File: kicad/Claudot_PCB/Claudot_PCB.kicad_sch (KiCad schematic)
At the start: 56 parts, among them J1 TYPE-C-31-M-12, SW1 SW_Push, SW10 SW_Push, SW11 SW_Push, SW12 RotaryEncoder, SW2 SW_Push, SW3 SW_Push, SW4 SW_Push, SW5 SW_Push, SW6 SW_Push, SW7 SW_Push, SW8 SW_Push, SW9 SW_Push, U1 RP2040, U2 W25Q16JVUXIQ, U3 AP2112K-3.3, Y1 12MHz

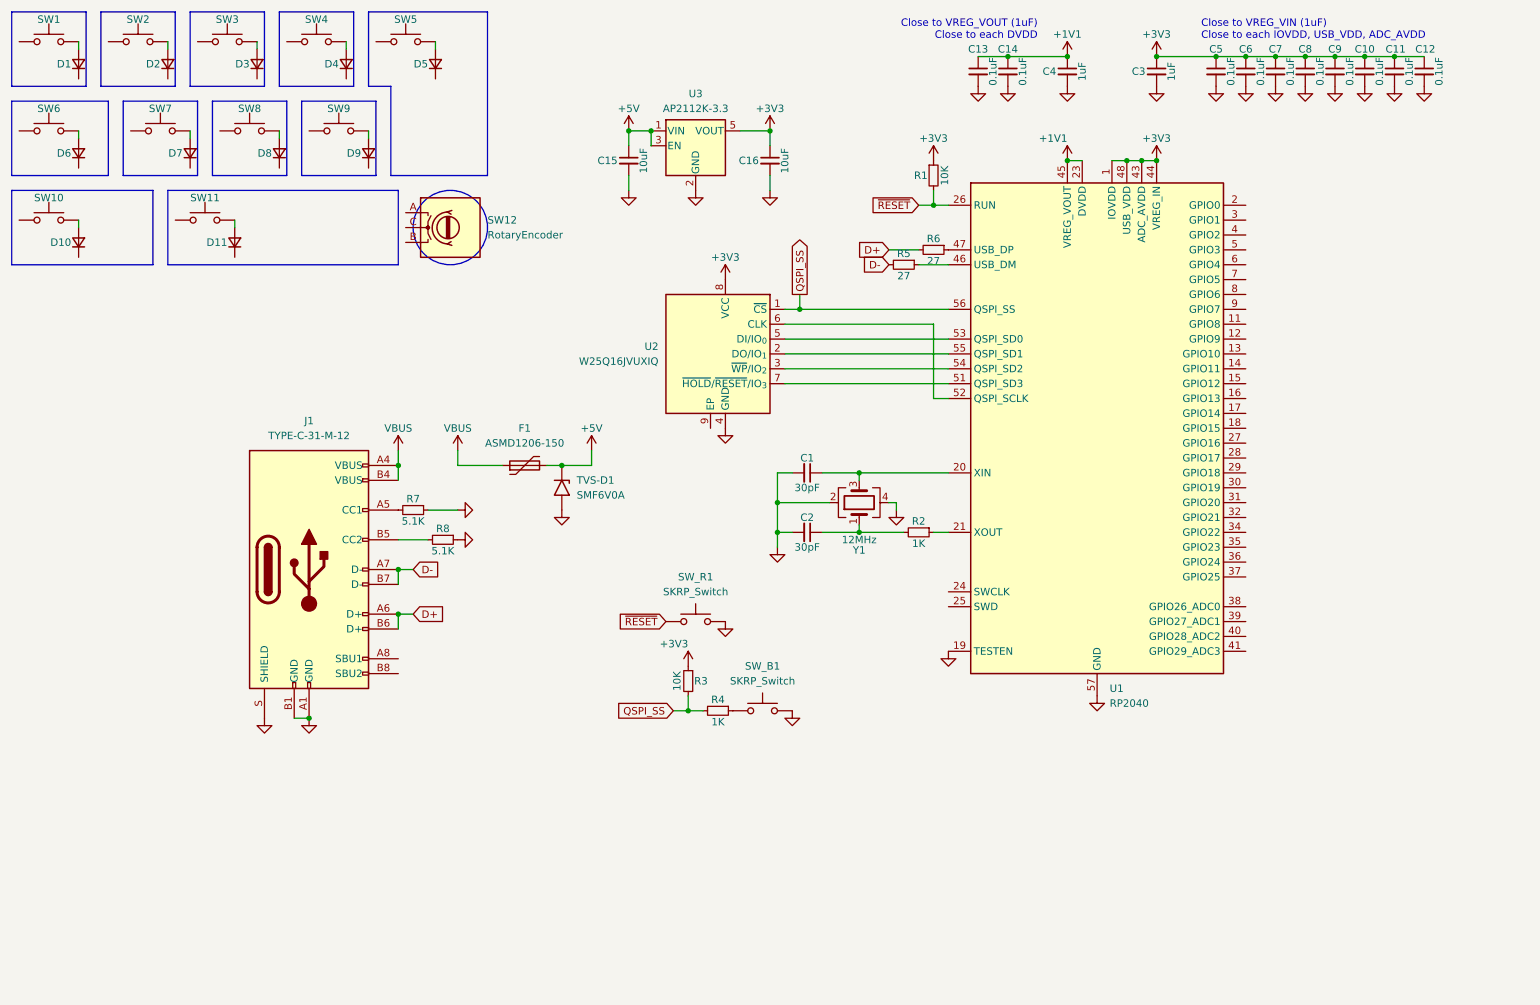
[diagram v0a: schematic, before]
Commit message: Update schematic and pcb
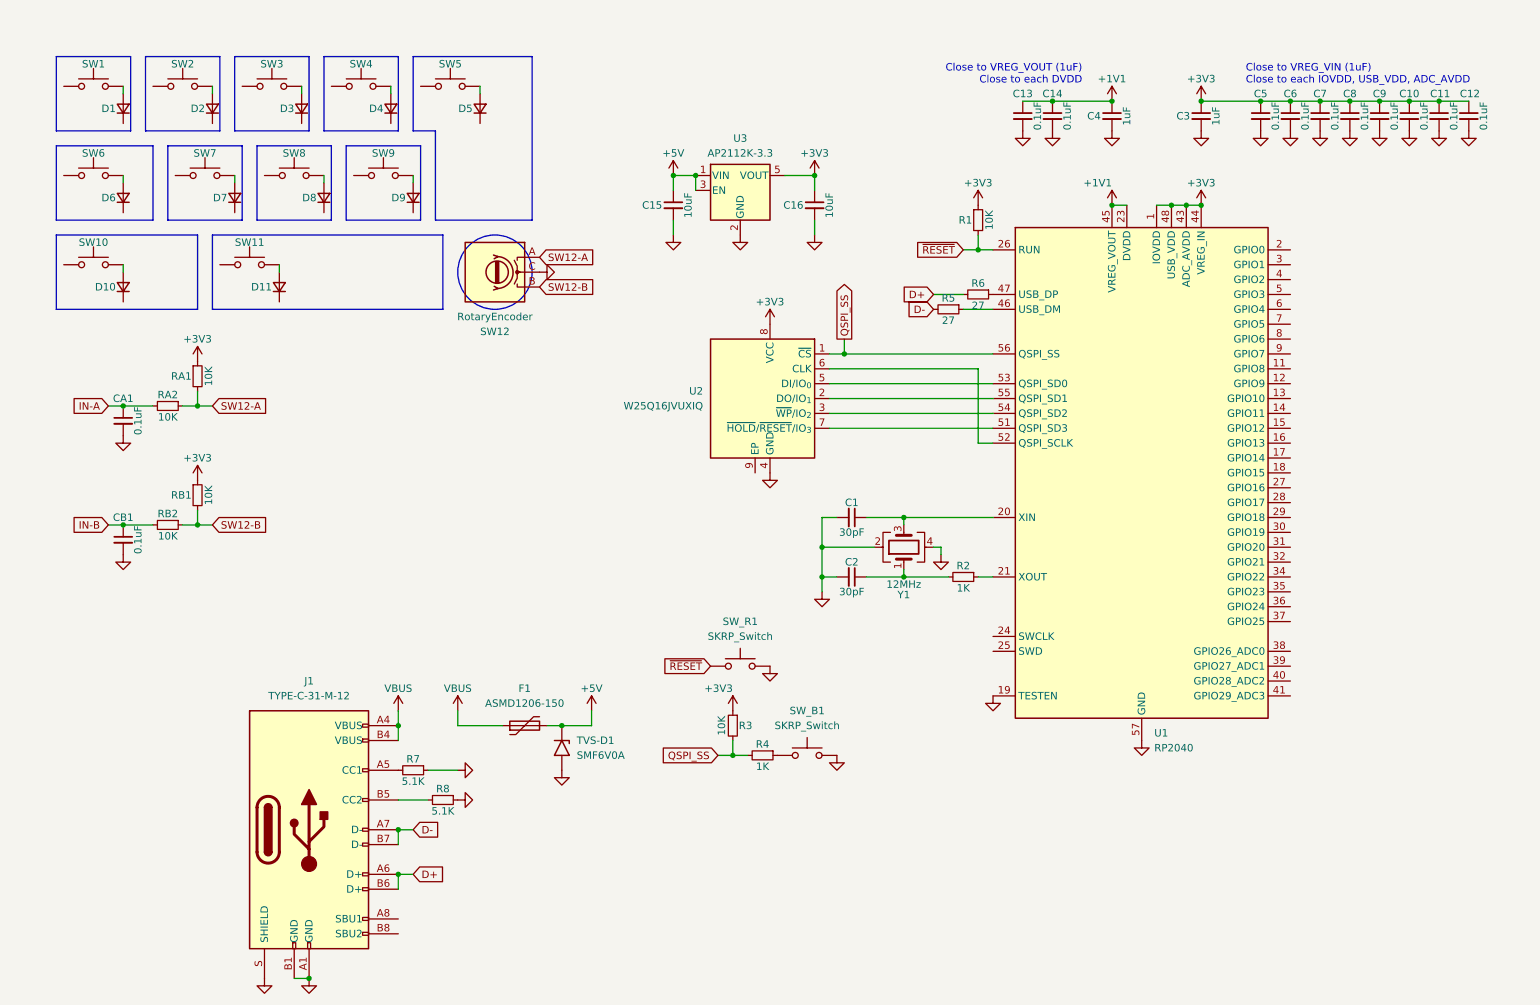
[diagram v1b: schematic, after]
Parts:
- added CA1, CB1: 0.1uF, Library:C_0402, symbol Device:C_Small
- added RA1, RA2, RB1, RB2: 10K, Library:R_0402, symbol Device:R_Small
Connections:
- net +3V3: now also RA1.1, RB1.1
- net GND: now also SW12.C, CA1.2, CB1.2
- net SW12-A: now reaches SW12.A
- net SW12-A: now also RA1.2, RA2.1
- net SW12-B: now reaches SW12.B
- net SW12-B: now also RB1.2, RB2.1
- new net IN-A: CA1.1, RA2.2
- new net IN-B: CB1.1, RB2.2
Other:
- moved on the sheet: C1, C10, C11, C12, C13, C14, C15, C16, C2, C3, C4, C5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

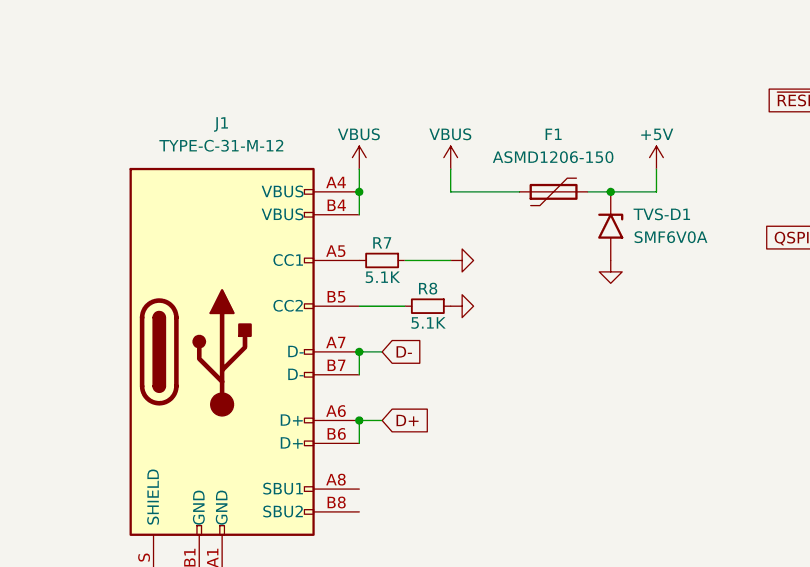
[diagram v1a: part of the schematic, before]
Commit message: Update schematic and pcb
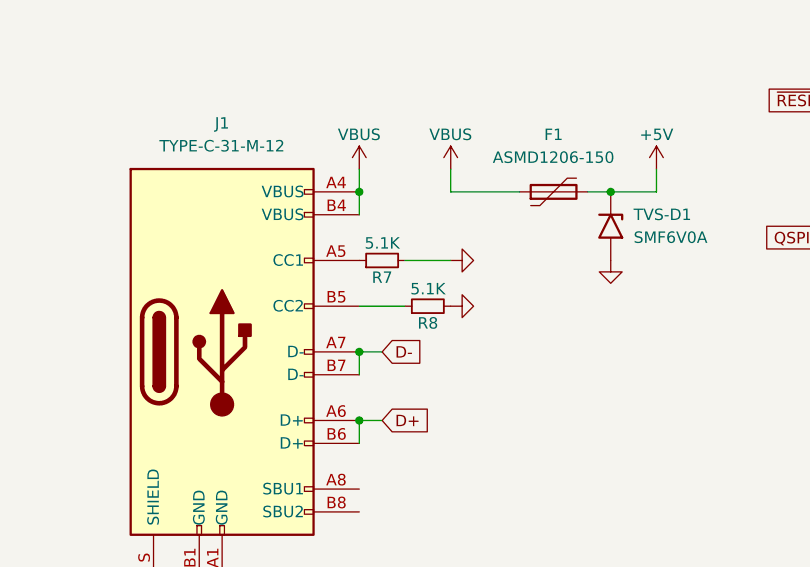
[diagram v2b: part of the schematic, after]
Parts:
- F1: footprint Fuse:Fuse_1206_3216Metric -> Library:F_1206
- TVS-D1: footprint Diode_SMD:D_SMF -> Library:SMF6.0A; LCSC (none) -> C178260
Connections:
- net GND: now also R7.2, R8.2; no longer R7.1, R8.1
- net at J1.A5 (CC1): now also R7.1; no longer R7.2
- net at J1.B5 (CC2): now also R8.1; no longer R8.2
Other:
- moved on the sheet: R7, R8
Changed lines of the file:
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@@
 			)
 		)
-		(property "Footprint" "Diode_SMD:D_SMF"
+		(property "Footprint" "Library:SMF6.0A"
 			(at 106.68 143.51 0)
 			(effects
@@
 			)
 		)
-		(property "Datasheet" "https://www.vishay.com/doc?85881"
+		(property "Datasheet" "~"
 			(at 111.76 142.24 0)
 			(effects
@@
 			)
 		)
-		(property "Description" "200W unidirectional Transil Transient Voltage Suppressor, 6Vrwm, SMF"
+		(property "Description" ""
 			(at 111.76 143.51 0)
 			(effects
@@
 			)
 		)
+		(property "LCSC" "C178260"
+			(at 111.76 143.51 90)
+			(effects
+				(font
+					(size 1.27 1.27)
+				)
+				(hide yes)
+			)
+		)
 		(pin "1"
 		)
@@
 	(symbol
 		(lib_id "Device:R_Small")
-		(at 86.36 147.32 270)
+		(at 86.36 147.32 90)
 		(unit 1)
 		(exclude_from_sim no)
@@
 		(dnp no)
 		(property "Reference" "R7"
-			(at 86.36 145.415 90)
+			(at 86.36 149.225 90)
 			(effects
 				(font
@@
 		)
 		(property "Value" "5.1K"
-			(at 86.36 149.225 90)
+			(at 86.36 145.415 90)
 			(effects
 				(font
@@
 			)
 		)
-		(property "Footprint" "Fuse:Fuse_1206_3216Metric"
+		(property "Footprint" "Library:F_1206"
 			(at 110.49 138.43 0)
 			(effects
@@
 	(symbol
 		(lib_id "Device:R_Small")
-		(at 91.44 152.4 270)
+		(at 91.44 152.4 90)
 		(unit 1)
 		(exclude_from_sim no)
@@
 		(dnp no)
 		(property "Reference" "R8"
-			(at 91.44 150.495 90)
+			(at 91.44 154.305 90)
 			(effects
 				(font
@@
 		)
 		(property "Value" "5.1K"
-			(at 91.44 154.305 90)
+			(at 91.44 150.495 90)
 			(effects
 				(font

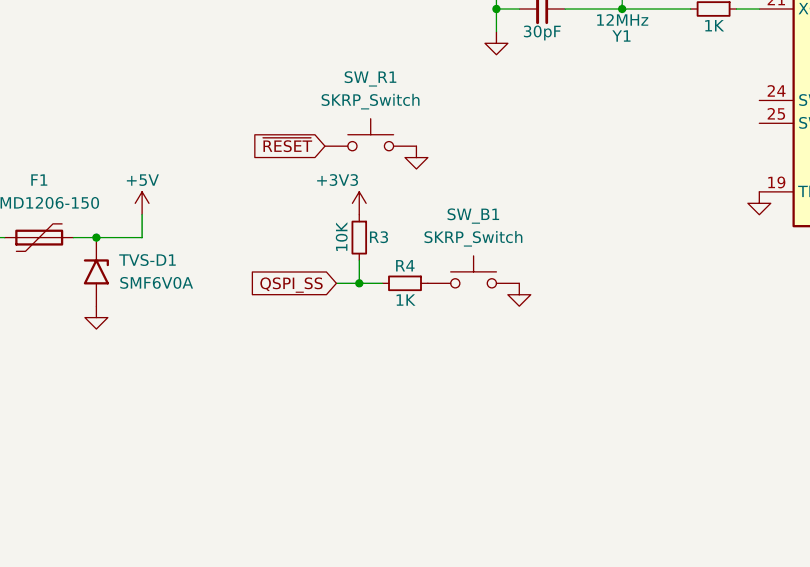
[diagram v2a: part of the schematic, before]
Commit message: Update schematic and pcb
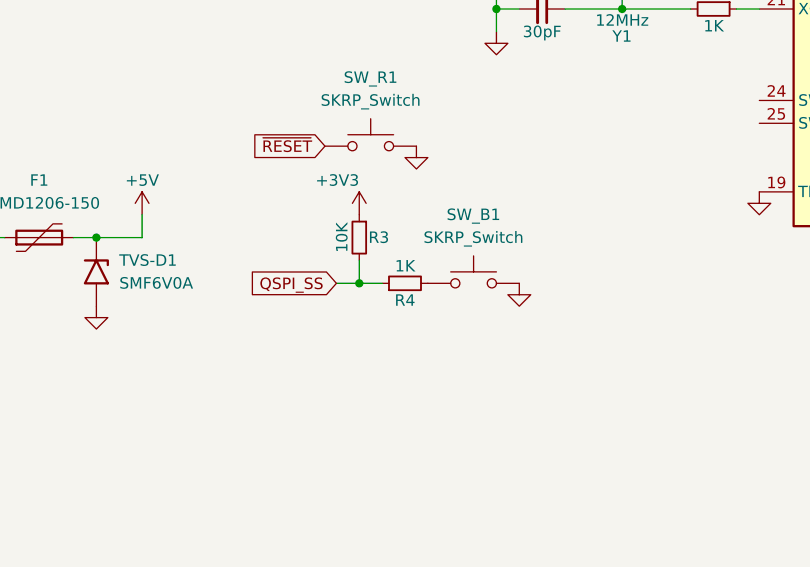
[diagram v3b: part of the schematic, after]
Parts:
- R3, R4: footprint Resistor_SMD:R_0402_1005Metric -> Library:R_0402
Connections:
- net QSPI_SS: now also R4.1; no longer R4.2
- net at SW_B1.1, SW_B1.2: now also R4.2; no longer R4.1
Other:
- moved on the sheet: R4
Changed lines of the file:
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@@
 			)
 		)
-		(property "Footprint" "Resistor_SMD:R_0402_1005Metric"
+		(property "Footprint" "Library:R_0402"
 			(at 140.97 139.7 0)
 			(effects
@@
 	(symbol
 		(lib_id "Device:R_Small")
-		(at 146.05 144.78 270)
+		(at 146.05 144.78 90)
 		(unit 1)
 		(exclude_from_sim no)
@@
 		(dnp no)
 		(property "Reference" "R4"
-			(at 146.05 142.875 90)
+			(at 146.05 146.685 90)
 			(effects
 				(font
@@
 		)
 		(property "Value" "1K"
-			(at 146.05 146.685 90)
+			(at 146.05 142.875 90)
 			(effects
 				(font
@@
 			)
 		)
-		(property "Footprint" "Resistor_SMD:R_0402_1005Metric"
+		(property "Footprint" "Library:R_0402"
 			(at 146.05 144.78 0)
 			(effects

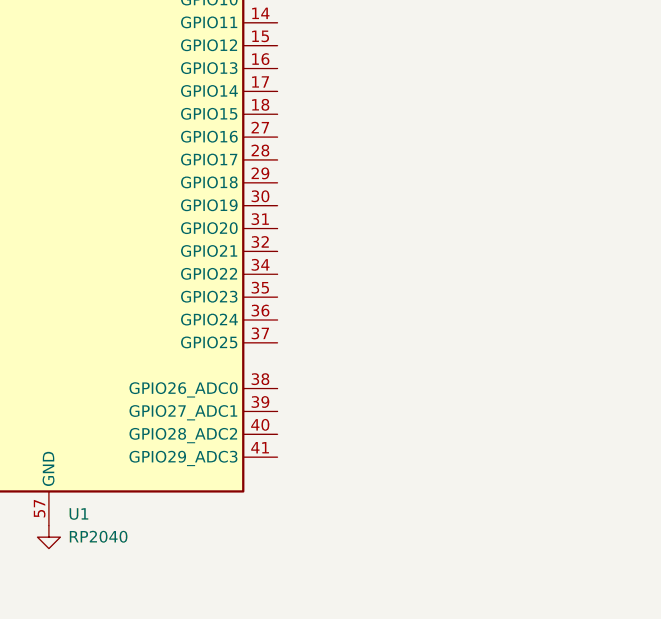
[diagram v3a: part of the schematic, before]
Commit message: Update schematic and pcb
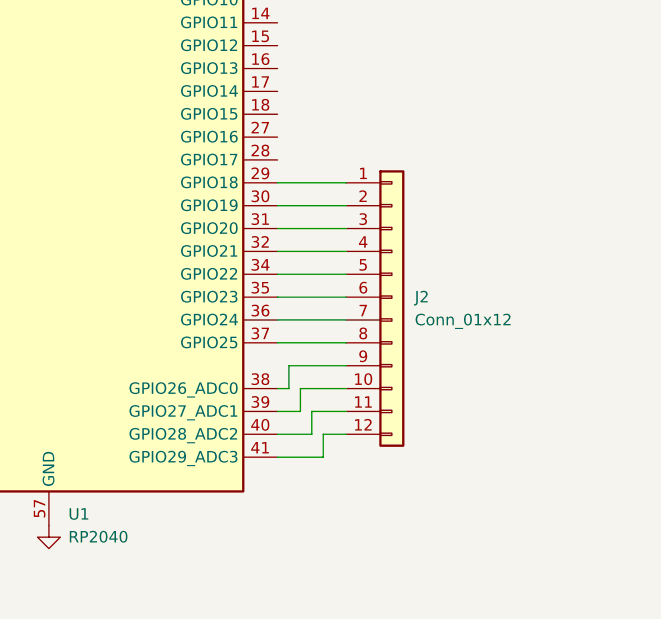
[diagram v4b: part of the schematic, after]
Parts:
- added J2: Conn_01x12, Library:AFC01-S12FCC-00, symbol Connector_Generic:Conn_01x12
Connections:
- net at U1.29 (GPIO18): now also J2.1 (Pin_1)
- net at U1.30 (GPIO19): now also J2.2 (Pin_2)
- net at U1.31 (GPIO20): now also J2.3 (Pin_3)
- net at U1.32 (GPIO21): now also J2.4 (Pin_4)
- net at U1.34 (GPIO22): now also J2.5 (Pin_5)
- net at U1.35 (GPIO23): now also J2.6 (Pin_6)
- net at U1.36 (GPIO24): now also J2.7 (Pin_7)
- net at U1.37 (GPIO25): now also J2.8 (Pin_8)
- net at U1.38 (GPIO26_ADC0): now also J2.9 (Pin_9)
- net at U1.39 (GPIO27_ADC1): now also J2.10 (Pin_10)
- net at U1.40 (GPIO28_ADC2): now also J2.11 (Pin_11)
- net at U1.41 (GPIO29_ADC3): now also J2.12 (Pin_12)
